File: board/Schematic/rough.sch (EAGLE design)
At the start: 2 parts

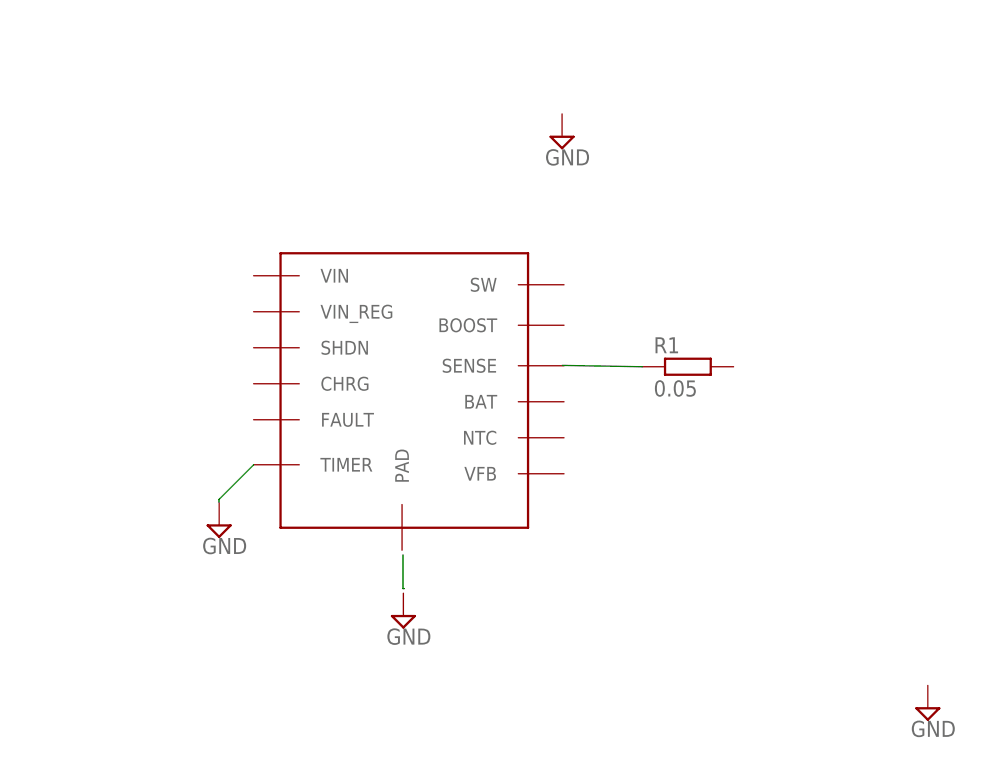
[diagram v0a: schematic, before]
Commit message: trying to fix docs glitch
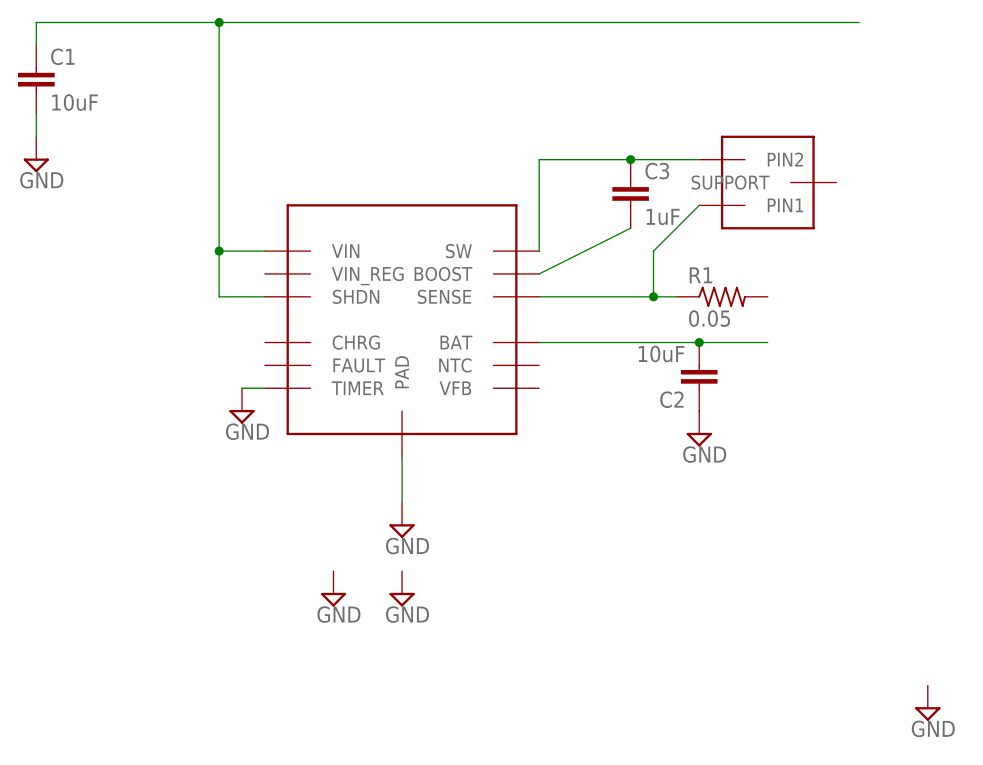
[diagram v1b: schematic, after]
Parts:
- added C1, C2: 10uF, capacitor-wima:C5/3.5
- added C3: 1uF, capacitor-wima:C5/3.5
- added INDUCTOR: INDUCTOR, Test:INDUCTOR
- R1: device rcl:R-EU_M3216 -> resistor:R-US_R1206
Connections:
- new net GND: C1.2, C2.1, U$1.PAD, U$1.TIMER
- new net N$2: C2.2, U$1.BAT
- new net N$3: INDUCTOR.PIN1, R1.1, U$1.SENSE
- new net N$4: C3.1, INDUCTOR.PIN2, U$1.SW
- new net N$5: C3.2, U$1.BOOST
- net N$1: now also C1.1, U$1.SHDN, U$1.VIN; no longer R1.1
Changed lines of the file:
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@@
 <setting verticaltext="up"/>
 </settings>
-<grid distance="0.05" unitdist="mm" unit="mm" style="lines" multiple="1" display="no" altdistance="0.01" altunitdist="inch" altunit="inch"/>
+<grid distance="0.1" unitdist="inch" unit="inch" style="lines" multiple="1" display="yes" altdistance="0.01" altunitdist="inch" altunit="inch"/>
 <layers>
 <layer number="1" name="Top" color="4" fill="1" visible="no" active="no"/>
@@
 <layer number="91" name="Nets" color="2" fill="1" visible="yes" active="yes"/>
 <layer number="92" name="Busses" color="1" fill="1" visible="yes" active="yes"/>
-<layer number="93" name="Pins" color="2" fill="1" visible="yes" active="yes"/>
+<layer number="93" name="Pins" color="2" fill="1" visible="no" active="yes"/>
 <layer number="94" name="Symbols" color="4" fill="1" visible="yes" active="yes"/>
 <layer number="95" name="Names" color="7" fill="1" visible="yes" active="yes"/>
@@
 </classes>
 <parts>
-<part name="U$1" library="Test" deviceset="LT3652" device=""/>
-<part name="R1" library="rcl" deviceset="R-EU_" device="M3216" value="0.05"/>
 <part name="SUPPLY1" library="supply2" deviceset="GND" device=""/>
-<part name="SUPPLY2" library="supply2" deviceset="GND" device=""/>
 <part name="SUPPLY3" library="supply2" deviceset="GND" device=""/>
 <part name="SUPPLY4" library="supply2" deviceset="GND" device=""/>
+<part name="C1" library="capacitor-wima" deviceset="C" device="5/3.5" value="10uF"/>
+<part name="C2" library="capacitor-wima" deviceset="C" device="5/3.5" value="10uF"/>
+<part name="C3" library="capacitor-wima" deviceset="C" device="5/3.5" value="1uF"/>
+<part name="INDUCTOR" library="Test" deviceset="INDUCTOR" device=""/>
+<part name="U$1" library="Test" deviceset="LT3652" device=""/>
+<part name="SUPPLY2" library="supply2" deviceset="GND" device=""/>
+<part name="SUPPLY5" library="supply2" deviceset="GND" device=""/>
+<part name="SUPPLY6" library="supply2" deviceset="GND" device=""/>
+<part name="SUPPLY7" library="supply2" deviceset="GND" device=""/>
+<part name="R1" library="resistor" deviceset="R-US_" device="R1206" value="0.05"/>
 </parts>
 <sheets>
@@
 </plain>
 <instances>
-<instance part="U$1" gate="G$2" x="53.34" y="48.26" rot="R270"/>
-<instance part="R1" gate="G$1" x="85.1" y="50.65"/>
-<instance part="SUPPLY1" gate="GND" x="33.02" y="33.02"/>
-<instance part="SUPPLY2" gate="GND" x="53.49" y="22.95"/>
+<instance part="SUPPLY1" gate="GND" x="12.7" y="73.66"/>
 <instance part="SUPPLY3" gate="GND" x="111.76" y="12.7"/>
-<instance part="SUPPLY4" gate="GND" x="71.12" y="76.2"/>
+<instance part="SUPPLY4" gate="GND" x="35.56" y="45.72"/>
+<instance part="C1" gate="G$1" x="12.7" y="83.82"/>
+<instance part="C2" gate="G$1" x="86.36" y="48.26" rot="R180"/>
+<instance part="C3" gate="G$1" x="78.74" y="71.12"/>
+<instance part="INDUCTOR" gate="G$1" x="93.98" y="71.12" rot="R90"/>
+<instance part="U$1" gate="G$2" x="53.34" y="55.88" rot="R270"/>
+<instance part="SUPPLY2" gate="GND" x="53.34" y="33.02"/>
+<instance part="SUPPLY5" gate="GND" x="53.34" y="25.4"/>
+<instance part="SUPPLY6" gate="GND" x="45.72" y="25.4"/>
+<instance part="SUPPLY7" gate="GND" x="86.36" y="43.18"/>
+<instance part="R1" gate="G$1" x="88.9" y="58.42"/>
 </instances>
 <busses>
@@
 <net name="N$1" class="0">
 <segment>
-<pinref part="R1" gate="G$1" pin="1"/>
-<wire x1="71.12" y1="50.8" x2="80.02" y2="50.65" width="0.1524" layer="91"/>
+<wire x1="12.7" y1="88.9" x2="33.02" y2="88.9" width="0.1524" layer="91"/>
+<pinref part="C1" gate="G$1" pin="1"/>
+<wire x1="33.02" y1="88.9" x2="104.14" y2="88.9" width="0.1524" layer="91"/>
+<wire x1="12.7" y1="86.36" x2="12.7" y2="88.9" width="0.1524" layer="91"/>
+<wire x1="33.02" y1="88.9" x2="33.02" y2="63.5" width="0.1524" layer="91"/>
+<junction x="33.02" y="88.9"/>
+<pinref part="U$1" gate="G$2" pin="SHDN"/>
+<wire x1="33.02" y1="63.5" x2="33.02" y2="58.42" width="0.1524" layer="91"/>
+<wire x1="33.02" y1="58.42" x2="38.1" y2="58.42" width="0.1524" layer="91"/>
+<pinref part="U$1" gate="G$2" pin="VIN"/>
+<wire x1="38.1" y1="63.5" x2="33.02" y2="63.5" width="0.1524" layer="91"/>
+<junction x="33.02" y="63.5"/>
+</segment>
+</net>
+<net name="GND" class="0">
+<segment>
+<pinref part="SUPPLY4" gate="GND" pin="GND"/>
+<pinref part="U$1" gate="G$2" pin="TIMER"/>
+<wire x1="35.56" y1="48.26" x2="38.1" y2="48.26" width="0.1524" layer="91"/>
+</segment>
+<segment>
+<pinref part="SUPPLY1" gate="GND" pin="GND"/>
+<pinref part="C1" gate="G$1" pin="2"/>
+<wire x1="12.7" y1="76.2" x2="12.7" y2="78.74" width="0.1524" layer="91"/>
+</segment>
+<segment>
+<pinref part="U$1" gate="G$2" pin="PAD"/>
+<pinref part="SUPPLY2" gate="GND" pin="GND"/>
+<wire x1="53.34" y1="40.64" x2="53.34" y2="35.56" width="0.1524" layer="91"/>
+</segment>
+<segment>
+<pinref part="C2" gate="G$1" pin="1"/>
+<pinref part="SUPPLY7" gate="GND" pin="GND"/>
 </segment>
 </net>
 <net name="N$2" class="0">
 <segment>
-<wire x1="33" y1="35.6" x2="33" y2="35.9" width="0.1524" layer="91"/>
-<wire x1="33" y1="35.9" x2="36.85" y2="39.75" width="0.1524" layer="91"/>
+<pinref part="U$1" gate="G$2" pin="BAT"/>
+<wire x1="68.58" y1="53.34" x2="86.36" y2="53.34" width="0.1524" layer="91"/>
+<pinref part="C2" gate="G$1" pin="2"/>
+<wire x1="86.36" y1="53.34" x2="93.98" y2="53.34" width="0.1524" layer="91"/>
+<junction x="86.36" y="53.34"/>
 </segment>
 </net>
 <net name="N$3" class="0">
 <segment>
-<wire x1="53.6" y1="26" x2="53.45" y2="26" width="0.1524" layer="91"/>
-<wire x1="53.45" y1="26" x2="53.45" y2="29.75" width="0.1524" layer="91"/>
+<pinref part="U$1" gate="G$2" pin="SENSE"/>
+<pinref part="R1" gate="G$1" pin="1"/>
+<wire x1="68.58" y1="58.42" x2="81.28" y2="58.42" width="0.1524" layer="91"/>
+<pinref part="INDUCTOR" gate="G$1" pin="PIN1"/>
+<wire x1="81.28" y1="58.42" x2="83.82" y2="58.42" width="0.1524" layer="91"/>
+<wire x1="86.36" y1="68.58" x2="81.28" y2="63.5" width="0.1524" layer="91"/>
+<wire x1="81.28" y1="63.5" x2="81.28" y2="58.42" width="0.1524" layer="91"/>
+<junction x="81.28" y="58.42"/>
 </segment>
 </net>
+<net name="N$4" class="0">
+<segment>
+<pinref part="U$1" gate="G$2" pin="SW"/>
+<pinref part="C3" gate="G$1" pin="1"/>
+<wire x1="68.58" y1="63.5" x2="68.58" y2="73.66" width="0.1524" layer="91"/>
+<wire x1="68.58" y1="73.66" x2="78.74" y2="73.66" width="0.1524" layer="91"/>
+<pinref part="INDUCTOR" gate="G$1" pin="PIN2"/>
+<wire x1="78.74" y1="73.66" x2="86.36" y2="73.66" width="0.1524" layer="91"/>
+<junction x="78.74" y="73.66"/>
+</segment>
+</net>
+<net name="N$5" class="0">
+<segment>
+<pinref part="U$1" gate="G$2" pin="BOOST"/>
+<pinref part="C3" gate="G$1" pin="2"/>
+<wire x1="68.58" y1="60.96" x2="78.74" y2="66.04" width="0.1524" layer="91"/>
+</segment>
+</net>
